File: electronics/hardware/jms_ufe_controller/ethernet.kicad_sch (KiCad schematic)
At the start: 26 parts, among them J11 RJ45_Amphenol_RJMG1BD3B8K1ANR, U3 DP83848KSQ_NOPB

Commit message: UFE Rev 2 off to the board fab
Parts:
- U3: LCSC (none) -> C43593
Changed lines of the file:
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@@
       (effects (font (size 1.27 1.27)) (justify left) hide)
+    )
+    (property "LCSC" "C43593" (id 21) (at 171.45 38.1 0)
+      (effects (font (size 1.27 1.27)) hide)
     )
     (pin "1")

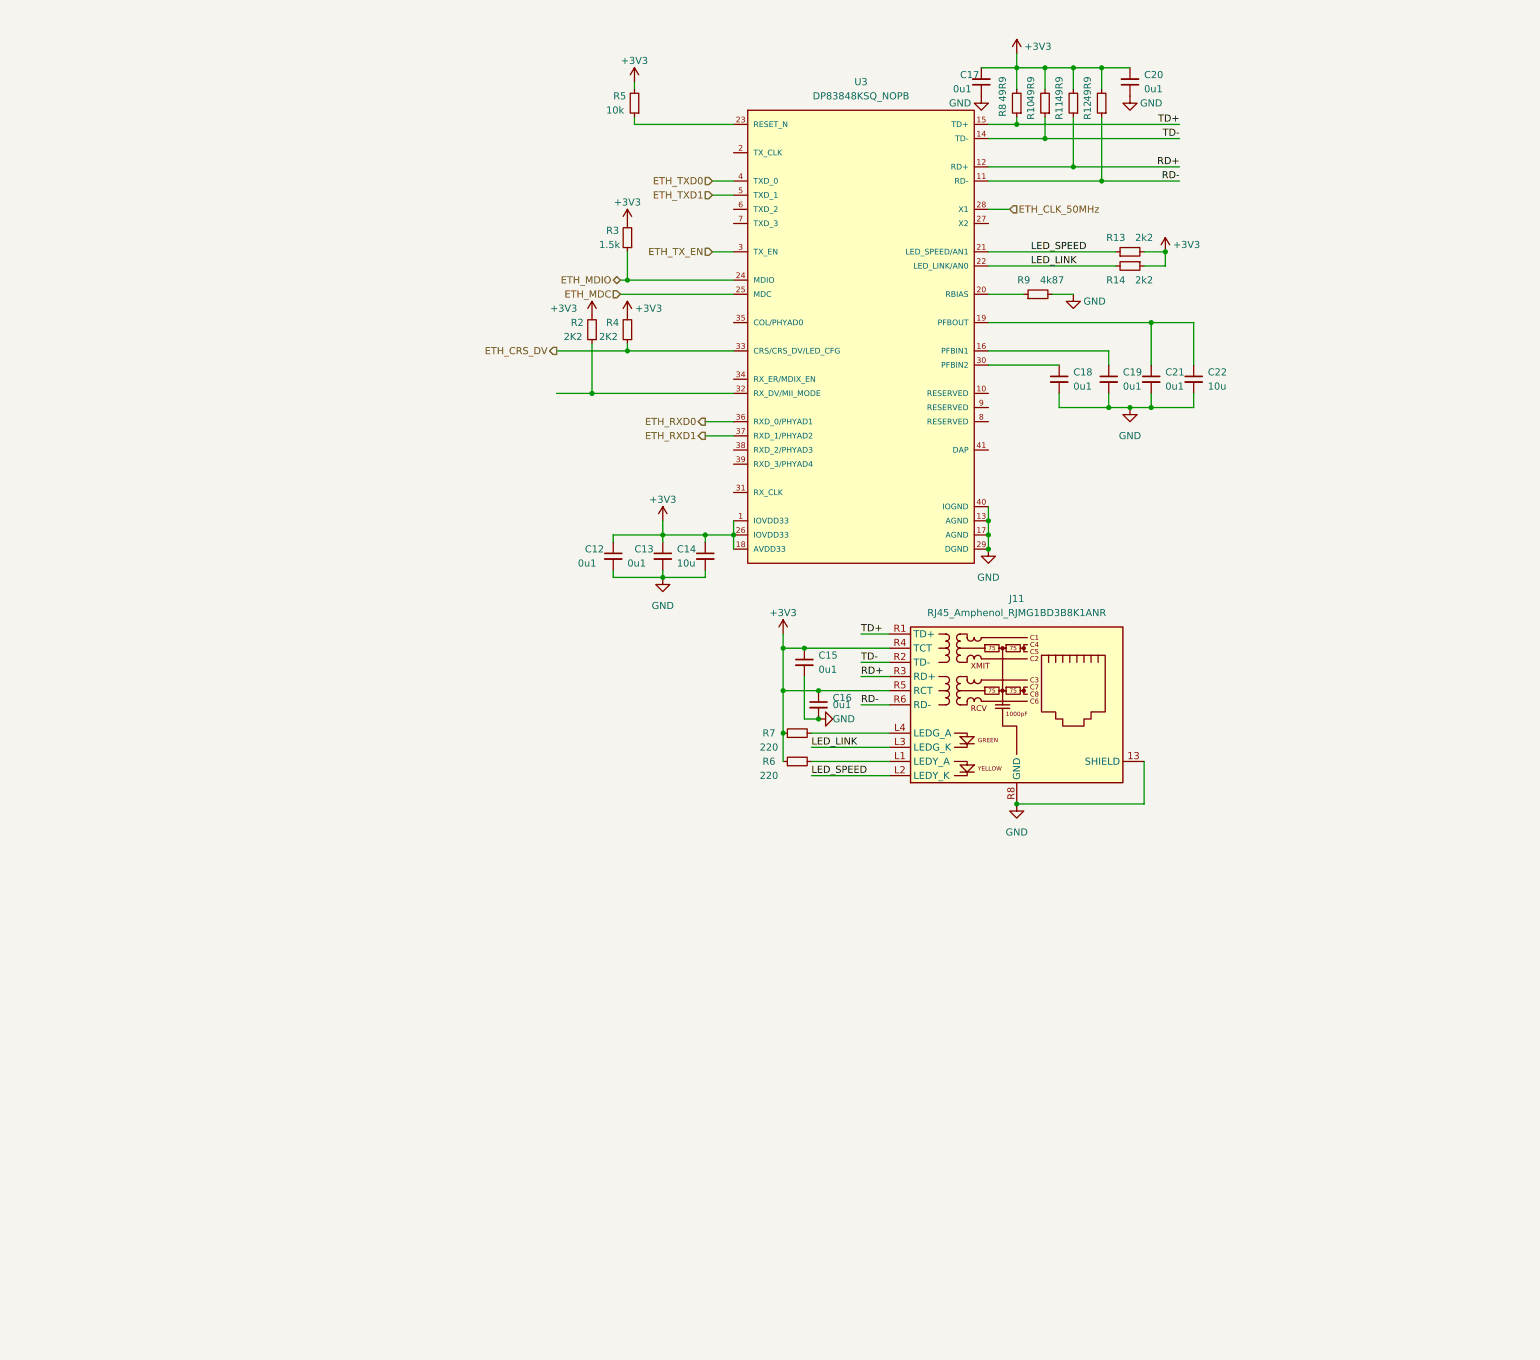
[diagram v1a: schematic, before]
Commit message: UFE Rev 3 - first try
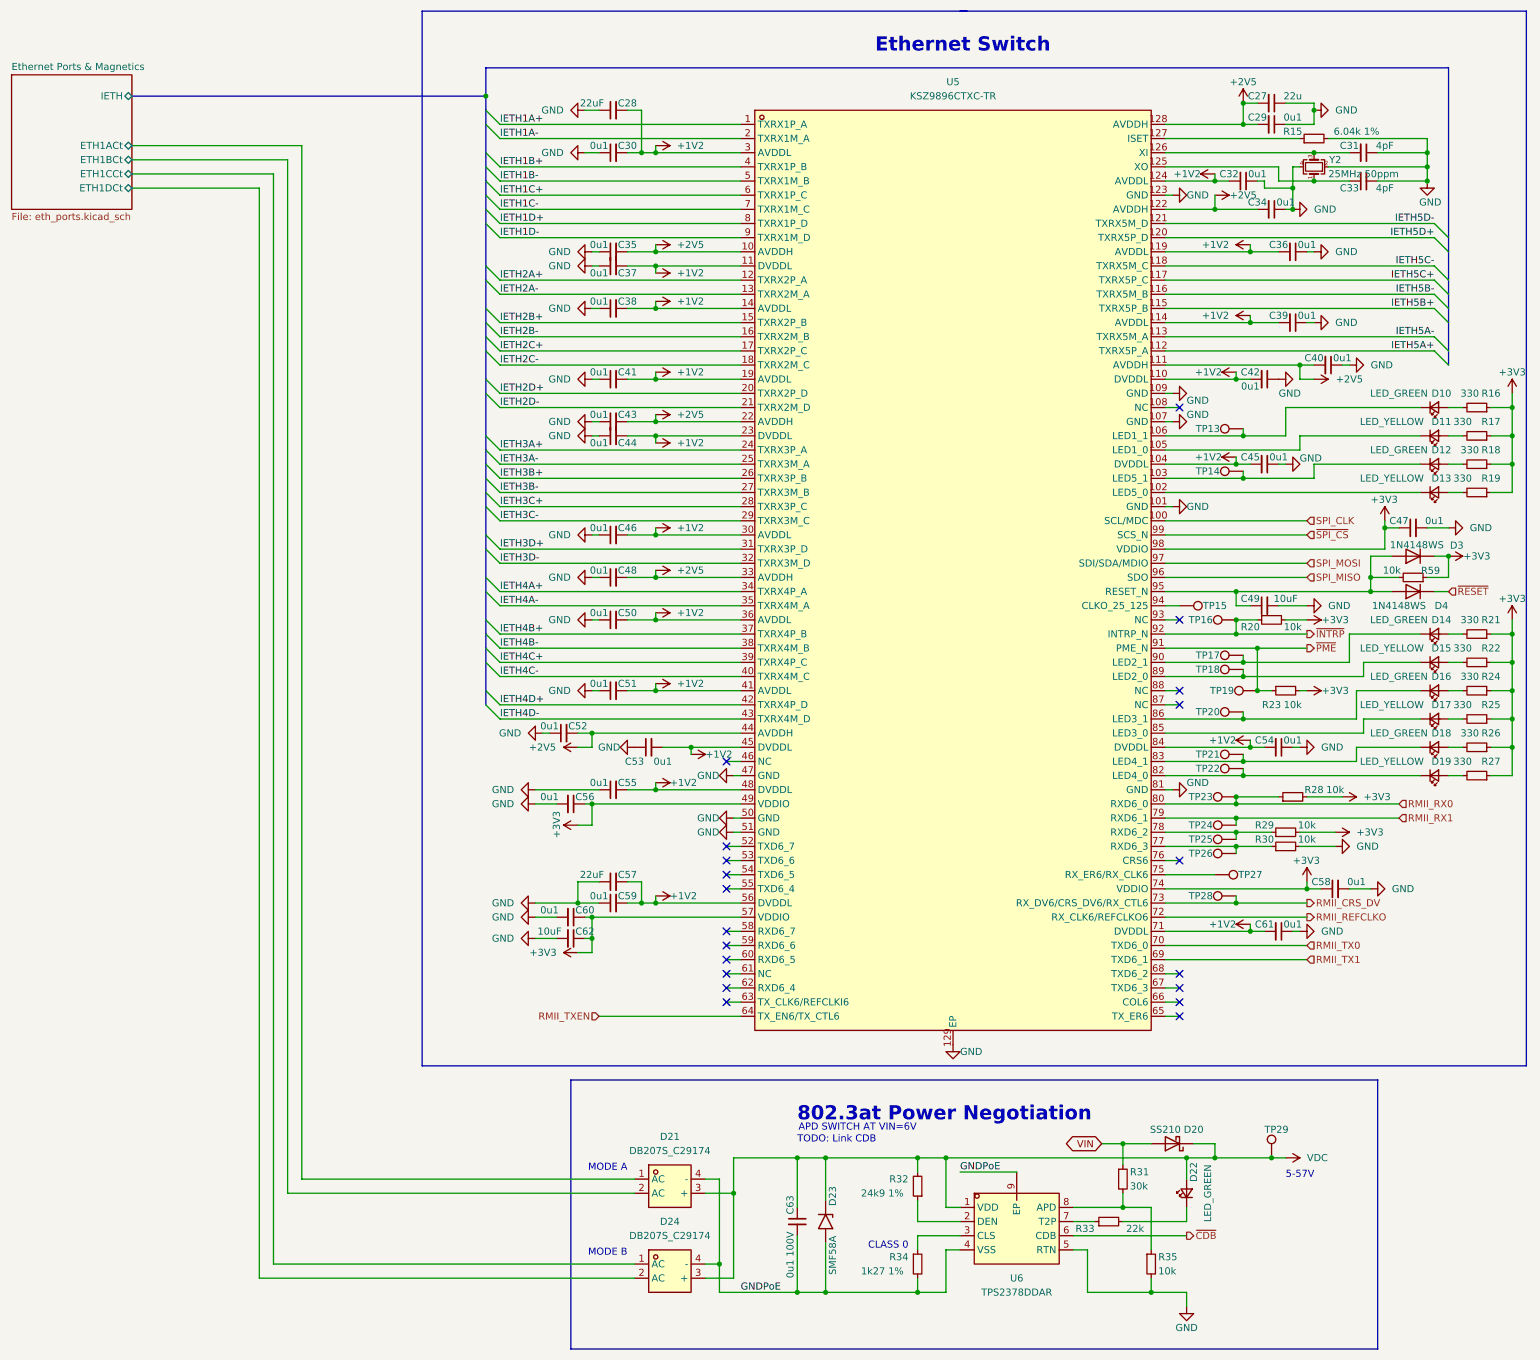
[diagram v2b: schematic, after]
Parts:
- removed C12, C13, C15, C16, C17, C18, C19, C20, C21: 0u1, Capacitor_SMD:C_0402_1005Metric, symbol Device:C_Small
- removed C14, C22: 10u, Capacitor_SMD:C_0402_1005Metric, symbol Device:C_Small
- removed J11: RJ45_Amphenol_RJMG1BD3B8K1ANR, Connector_RJ:RJ45_Amphenol_RJMG1BD3B8K1ANR, symbol Connector:RJ45_Amphenol_RJMG1BD3B8K1ANR
- removed R10, R11, R12, R8: 49R9, Resistor_SMD:R_0402_1005Metric, symbol Device:R_Small
- removed R13, R14: 2k2, Resistor_SMD:R_0402_1005Metric, symbol Device:R_Small
- removed R2, R4: 2K2, Resistor_SMD:R_0402_1005Metric, symbol Device:R_Small
- removed R3: 1.5k, Resistor_SMD:R_0402_1005Metric, symbol Device:R_Small
- removed R5: 10k, Resistor_SMD:R_0402_1005Metric, symbol Device:R_Small
- removed R6, R7: 220, Resistor_SMD:R_0402_1005Metric, symbol Device:R_Small
- removed R9: 4k87, Resistor_SMD:R_0402_1005Metric, symbol Device:R_Small
- removed U3: DP83848KSQ_NOPB, Project:Texas_Instruments-DP83848KSQ_NOPB-0, symbol TI_ETH:DP83848KSQ_NOPB
- added C27: 22u, Capacitor_SMD:C_0402_1005Metric, symbol Device:C_Small
- added C28, C57: 22uF, Capacitor_SMD:C_0402_1005Metric, symbol Device:C_Small
- added C29, C30, C32, C34, C35, C36, C37, C38, C39, C40, C41, C42, C43, C44, C45, C46, C47, C48, C50, C51, C52, C53, C54, C55, C56, C58, C59, C60, C61: 0u1, Capacitor_SMD:C_0402_1005Metric, symbol Device:C_Small
- added C31, C33: 4pF, Capacitor_SMD:C_0402_1005Metric, symbol Device:C_Small
- added C49, C62: 10uF, Capacitor_SMD:C_0402_1005Metric, symbol Device:C_Small
- added C63: 0u1 100V, Capacitor_SMD:C_0805_2012Metric, symbol Device:C_Small
- added D10, D12, D14, D16, D18, D22: LED_GREEN, LED_SMD:LED_0603_1608Metric, symbol Device:LED_Small
- added D11, D13, D15, D17, D19: LED_YELLOW, LED_SMD:LED_0603_1608Metric, symbol Device:LED_Small
- added D20: SS210, Diode_SMD:D_SMA, symbol Device:D_Schottky
- added D21, D24: DB207S_C29174, DB207S:DBS_L8.4-W6.4-P5.10-LS10.2-TL, symbol DB207S:DB207S_C29174
- added D23: SMF58A, Diode_SMD:D_SMF, symbol Diode:SMF58A
- added D3, D4: 1N4148WS, Diode_SMD:D_SOD-323, symbol Diode:1N4148WS
- added R15: 6.04k 1%, Resistor_SMD:R_0402_1005Metric, symbol Device:R_Small
- added R16, R17, R18, R19, R21, R22, R24, R25, R26, R27: 330, Resistor_SMD:R_0402_1005Metric, symbol Device:R_Small
- added R20, R23, R28, R29, R30, R35, R59: 10k, Resistor_SMD:R_0402_1005Metric, symbol Device:R_Small
- added R31: 30k, Resistor_SMD:R_0402_1005Metric, symbol Device:R_Small
- added R32: 24k9 1%, Resistor_SMD:R_0402_1005Metric, symbol Device:R_Small
- added R33: 22k, Resistor_SMD:R_0402_1005Metric, symbol Device:R_Small
- added R34: 1k27 1%, Resistor_SMD:R_0402_1005Metric, symbol Device:R_Small
- added TP13, TP14, TP15, TP16, TP17, TP18, TP19, TP20, TP21, TP22, TP23, TP24, TP25, TP26, TP27, TP28, TP29: TestPoint, TestPoint:TestPoint_Pad_1.5x1.5mm, symbol Connector:TestPoint
- added U5: KSZ9896CTXC-TR, KSZ9896CTXC-TR:TQFP-128_L14.0-W14.0-P0.40-LS16.0-BL-EP, symbol KSZ9896CTXC-TR:KSZ9896CTXC-TR
- added U6: TPS2378DDAR, TPS2378DDAR:SO-8_L4.9-W3.9-P1.27-LS6.0-BL-EP, symbol TPS2378DDAR:TPS2378DDAR
- added Y2: 25MHz 50ppm, Crystal:Crystal_SMD_3225-4Pin_3.2x2.5mm, symbol Device:Crystal_GND24_Small
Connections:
- net +3V3: now also C47.1, C56.1, C58.1, C60.1, C62.1, D3.1 (K), R16.1, R17.1, R18.1, R19.1, R20.2, R21.1, R22.1, R23.2, R24.1, R25.1, R26.1, R27.1, R28.2, R29.2, R59.1, U5.49 (VDDIO), U5.57 (VDDIO), U5.74 (VDDIO), U5.98 (VDDIO)
- net GND: now also C27.1, C28.1, C29.1, C30.1, C31.1, C32.1, C33.2, C34.1, C35.1, C36.1, C37.1, C38.1, C39.1, C40.1, C41.1, C42.1, C43.1, C44.1, C45.1, C46.1, C47.2, C48.1, C49.2, C50.1, C51.1, C52.1, C53.1, C54.1, C55.1, C56.2, C57.1, C58.2, C59.1, C60.2, C61.1, C62.2, R15.2, R30.2, R35.2, U5.101 (GND), U5.107 (GND), U5.109 (GND), U5.123 (GND), U5.129 (EP), U5.47 (GND), U5.50 (GND), U5.51 (GND), U5.81 (GND), U6.5 (RTN), Y2.2, Y2.4
- new net: R31.2, R35.1, U6.8 (APD)
- new net: D14.1 (K), TP17.1, U5.90 (LED2_1)
- new net: D14.2 (A), R21.2
- new net: D18.1 (K), TP21.1, U5.83 (LED4_1)
- new net: D12.1 (K), TP14.1, U5.103 (LED5_1)
- new net: D13.1 (K), U5.102 (LED5_0)
- new net: D11.1 (K), U5.105 (LED1_0)
- new net: D10.1 (K), TP13.1, U5.106 (LED1_1)
- new net: C33.1, U5.125 (XO), Y2.1
- new net: C31.2, U5.126 (XI), Y2.3
- new net: R15.1, U5.127 (ISET)
- new net: TP27.1, U5.75 (RX_ER6/RX_CLK6)
- new net: R30.1, TP26.1, U5.77 (RXD6_3)
- new net: R29.1, TP25.1, U5.78 (RXD6_2)
- new net: D19.1 (K), TP22.1, U5.82 (LED4_0)
- new net: D17.1 (K), U5.85 (LED3_0)
- new net: D16.1 (K), TP20.1, U5.86 (LED3_1)
- new net: D15.1 (K), TP18.1, U5.89 (LED2_0)
- new net: TP15.1, U5.94 (CLKO_25_125)
- new net: C49.1, D3.2 (A), D4.2 (A), R59.2, U5.95 (RESET_N)
- new net: D12.2 (A), R18.2
- new net: D15.2 (A), R22.2
- new net: R33.1, U6.7 (T2P)
- new net: D22.1 (K), R33.2
- new net: D18.2 (A), R26.2
- new net: D19.2 (A), R27.2
- new net: D13.2 (A), R19.2
- new net: R32.1, U6.2 (DEN)
- new net: R34.1, U6.3 (CLS)
- new net: D11.2 (A), R17.2
- new net: D16.2 (A), R24.2
- new net: D17.2 (A), R25.2
- new net: D10.2 (A), R16.2
- new net +1V2: C28.2, C30.2, C32.2, C36.2, C37.2, C38.2, C39.2, C41.2, C42.2, C44.2, C45.2, C46.2, C50.2, C51.2, C53.2, C54.2, C55.2, C57.2, C59.2, C61.2, U5.104 (DVDDL), U5.11 (DVDDL), U5.110 (DVDDL), U5.114 (AVDDL), U5.119 (AVDDL), U5.124 (AVDDL), U5.14 (AVDDL), U5.19 (AVDDL), U5.23 (DVDDL), U5.3 (AVDDL), U5.30 (AVDDL), U5.36 (AVDDL), U5.41 (AVDDL), U5.45 (DVDDL), U5.48 (DVDDL), U5.56 (DVDDL), U5.71 (DVDDL), U5.84 (DVDDL)
- new net +2V5: C27.2, C29.2, C34.2, C35.2, C40.2, C43.2, C48.2, C52.2, U5.10 (AVDDH), U5.111 (AVDDH), U5.122 (AVDDH), U5.128 (AVDDH), U5.22 (AVDDH), U5.33 (AVDDH), U5.44 (AVDDH)
- new net Ethernet Ports & Magnetics/ETH1ACt: D21.1 (AC)
- new net Ethernet Ports & Magnetics/ETH1BCt: D21.2 (AC)
- new net Ethernet Ports & Magnetics/ETH1CCt: D24.1 (AC)
- new net Ethernet Ports & Magnetics/ETH1DCt: D24.2 (AC)
- new net GNDPoE: C63.2, D21.4 (-), D23.2 (A2), D24.4 (-), R34.2, U6.4 (VSS), U6.9 (EP)
- new net IETH1A+: U5.1 (TXRX1P_A)
- new net IETH1A-: U5.2 (TXRX1M_A)
- new net IETH1B+: U5.4 (TXRX1P_B)
- new net IETH1B-: U5.5 (TXRX1M_B)
- new net IETH1C+: U5.6 (TXRX1P_C)
- new net IETH1C-: U5.7 (TXRX1M_C)
- new net IETH1D+: U5.8 (TXRX1P_D)
- new net IETH1D-: U5.9 (TXRX1M_D)
- new net IETH2A+: U5.12 (TXRX2P_A)
- new net IETH2A-: U5.13 (TXRX2M_A)
- new net IETH2B+: U5.15 (TXRX2P_B)
- new net IETH2B-: U5.16 (TXRX2M_B)
- new net IETH2C+: U5.17 (TXRX2P_C)
- new net IETH2C-: U5.18 (TXRX2M_C)
- new net IETH2D+: U5.20 (TXRX2P_D)
- new net IETH2D-: U5.21 (TXRX2M_D)
- new net IETH3A+: U5.24 (TXRX3P_A)
- new net IETH3A-: U5.25 (TXRX3M_A)
- new net IETH3B+: U5.26 (TXRX3P_B)
- new net IETH3B-: U5.27 (TXRX3M_B)
- new net IETH3C+: U5.28 (TXRX3P_C)
- new net IETH3C-: U5.29 (TXRX3M_C)
- new net IETH3D+: U5.31 (TXRX3P_D)
- new net IETH3D-: U5.32 (TXRX3M_D)
- new net IETH4A+: U5.34 (TXRX4P_A)
- new net IETH4A-: U5.35 (TXRX4M_A)
- new net IETH4B+: U5.37 (TXRX4P_B)
- new net IETH4B-: U5.38 (TXRX4M_B)
- new net IETH4C+: U5.39 (TXRX4P_C)
- new net IETH4C-: U5.40 (TXRX4M_C)
- new net IETH4D+: U5.42 (TXRX4P_D)
- new net IETH4D-: U5.43 (TXRX4M_D)
- new net IETH5A+: U5.112 (TXRX5P_A)
- new net IETH5A-: U5.113 (TXRX5M_A)
- new net IETH5B+: U5.115 (TXRX5P_B)
- new net IETH5B-: U5.116 (TXRX5M_B)
- new net IETH5C+: U5.117 (TXRX5P_C)
- new net IETH5C-: U5.118 (TXRX5M_C)
- new net IETH5D+: U5.120 (TXRX5P_D)
- new net IETH5D-: U5.121 (TXRX5M_D)
- new net RMII_CRS_DV: TP28.1, U5.73 (RX_DV6/CRS_DV6/RX_CTL6)
- new net RMII_REFCLKO: U5.72 (RX_CLK6/REFCLKO6)
- new net RMII_RX0: R28.1, TP23.1, U5.80 (RXD6_0)
- new net RMII_RX1: TP24.1, U5.79 (RXD6_1)
- new net RMII_TX0: U5.70 (TXD6_0)
- new net RMII_TX1: U5.69 (TXD6_1)
- new net RMII_TXEN: U5.64 (TX_EN6/TX_CTL6)
- new net SPI_CLK: U5.100 (SCL/MDC)
- new net SPI_MISO: U5.96 (SDO)
- new net SPI_MOSI: U5.97 (SDI/SDA/MDIO)
- new net VDC: C63.1, D20.1 (K), D21.3 (+), D22.2 (A), D23.1 (A1), D24.3 (+), R32.2, TP29.1, U6.1 (VDD)
- new net VIN: D20.2 (A), R31.1
- new net ~{CDB}: U6.6 (CDB)
- new net ~{INTRP}: R20.1, TP16.1, U5.92 (INTRP_N)
- new net ~{PME}: R23.1, TP19.1, U5.91 (PME_N)
- new net ~{RESET}: D4.1 (K)
- new net ~{SPI_CS}: U5.99 (SCS_N)
- no-connect marks 0 -> 20
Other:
- added sheet Ethernet Ports & Magnetics (eth_ports.kicad_sch)
- note added: "5-57V"
- note added: "802.3at Power Negotiation"
- note added: "APD SWITCH AT VIN=6V"
- note added: "CLASS 0"
- note added: "Ethernet Switch"
- note added: "MODE A"
- note added: "MODE B"
- note added: "TODO: Link CDB"
